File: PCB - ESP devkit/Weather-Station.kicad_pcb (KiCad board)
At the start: 2 copper layers, 61.5 x 50.5 mm, 28 parts, among them J1 Biruta, J10 Conn_01x19, J11 Conn_01x19, J2 Power, J3 BH1750-FVI, J4 BME280, J5 Pluviometro, J6 Anemometro, J8 Conn_01x02, J9 Conn_01x02, U1 AP1117-33

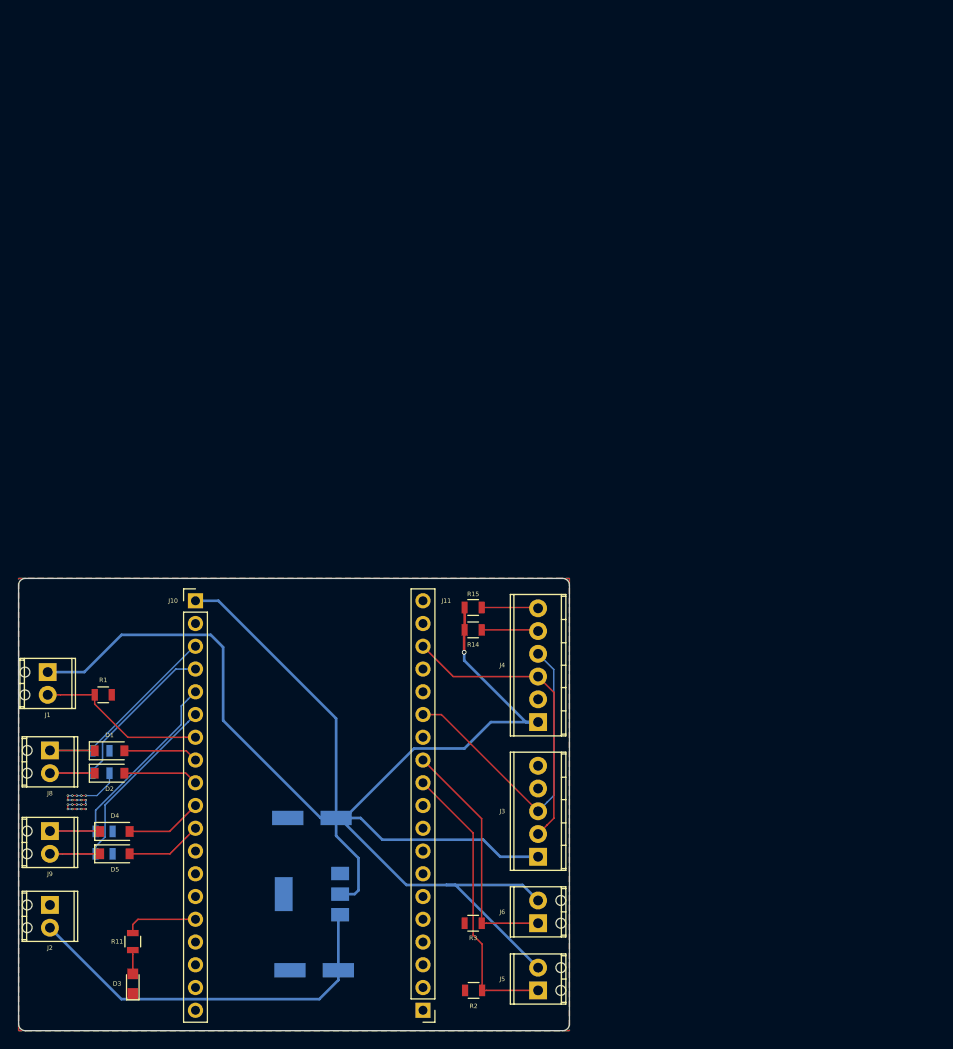
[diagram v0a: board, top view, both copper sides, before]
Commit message: Ajustando PCBs
Signed-off-by: Gustavo Costa <gustavocosta@ic.ufal.br>
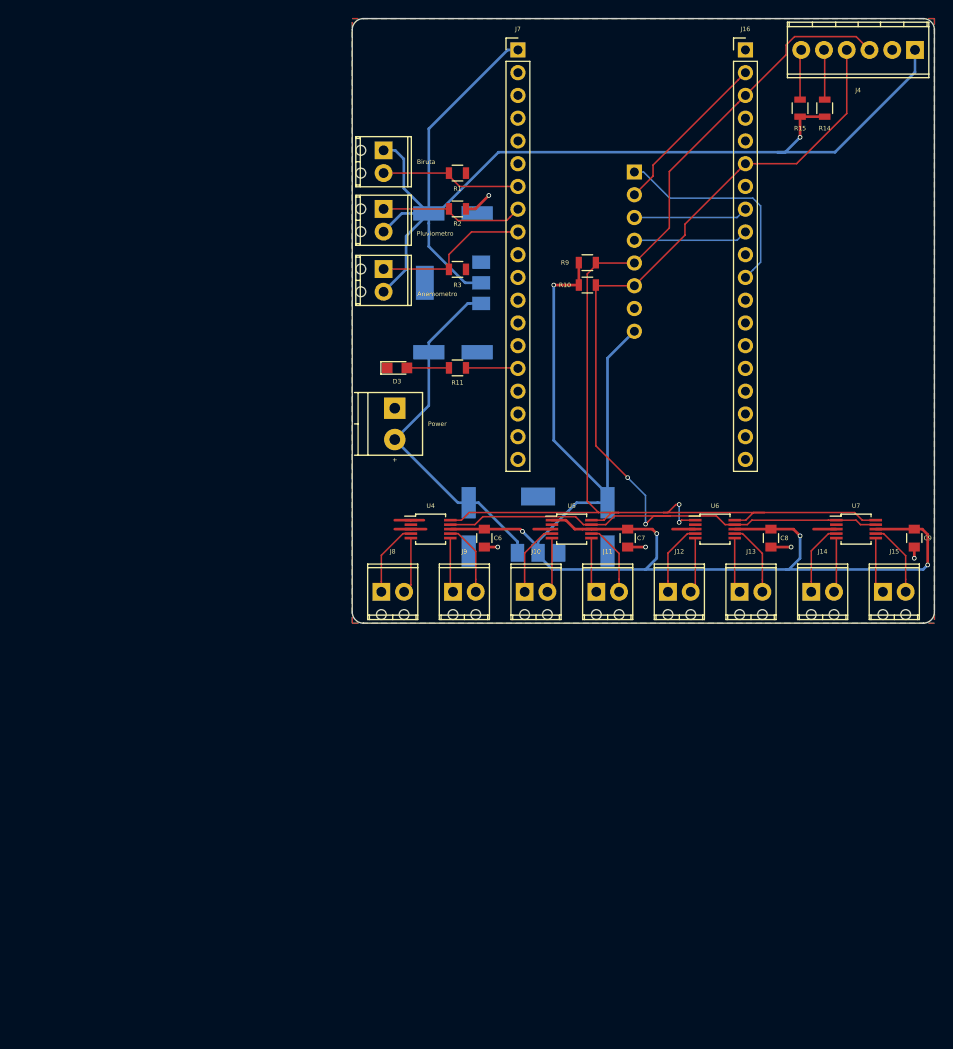
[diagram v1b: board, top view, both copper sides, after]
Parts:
- removed D1, D2, D4, D5: D, Diodes_SMD:D_SOD-123
- removed J1: Biruta, TerminalBlock_Phoenix:TerminalBlock_Phoenix_MPT-2.54mm_2pol
- removed J2: Power, TerminalBlock_Phoenix:TerminalBlock_Phoenix_MPT-2.54mm_2pol
- removed J5: Pluviometro, TerminalBlock_Phoenix:TerminalBlock_Phoenix_MPT-2.54mm_2pol
- removed J6: Anemometro, TerminalBlock_Phoenix:TerminalBlock_Phoenix_MPT-2.54mm_2pol
- removed R12, R13: 1.5K, Resistors_SMD:R_0805
- added Anemometro: Anemometro, TerminalBlock_Phoenix:TerminalBlock_Phoenix_MPT-2.54mm_2pol, F.Cu at (106.0, 55.5)
- added Biruta: Biruta, TerminalBlock_Phoenix:TerminalBlock_Phoenix_MPT-2.54mm_2pol, F.Cu at (106.0, 42.2)
- added C4: 22μF, Capacitors_SMD:CP_Elec_6.3x7.7, B.Cu at (115.5, 84.2)
- added C5: 22μF, Capacitors_SMD:CP_Elec_6.3x7.7, B.Cu at (131.0, 84.2)
- added C6: 0.1uF, Capacitors_SMD:C_0805, F.Cu at (117.2, 85.5)
- added C7: 0.1uF, Capacitors_SMD:C_0805, F.Cu at (133.2, 85.5)
- added C8: 0.1uF, Capacitors_SMD:C_0805, F.Cu at (149.2, 85.5)
- added C9: 0.1uF, Capacitors_SMD:C_0805, F.Cu at (165.2, 85.5)
- added J12: Conn_01x02, TerminalBlock_Phoenix:TerminalBlock_Phoenix_MPT-2.54mm_2pol, F.Cu at (137.8, 91.5)
- added J13: Conn_01x02, TerminalBlock_Phoenix:TerminalBlock_Phoenix_MPT-2.54mm_2pol, F.Cu at (145.8, 91.5)
- added J14: Conn_01x02, TerminalBlock_Phoenix:TerminalBlock_Phoenix_MPT-2.54mm_2pol, F.Cu at (153.8, 91.5)
- added J15: Conn_01x02, TerminalBlock_Phoenix:TerminalBlock_Phoenix_MPT-2.54mm_2pol, F.Cu at (161.8, 91.5)
- added J16: Conn_01x19, Pin_Headers:Pin_Header_Straight_1x19_Pitch2.54mm, F.Cu at (146.4, 31.0)
- added J7: Conn_01x19, Pin_Headers:Pin_Header_Straight_1x19_Pitch2.54mm, F.Cu at (121.0, 31.0)
- added Pluviometro: Pluviometro, TerminalBlock_Phoenix:TerminalBlock_Phoenix_MPT-2.54mm_2pol, F.Cu at (106.0, 48.8)
- added Power: Power, TerminalBlock_Phoenix:TerminalBlock_Phoenix_PT-3.5mm_2pol, F.Cu at (107.2, 71.0)
- added U3: AP1117-33, TO_SOT_Packages_SMD:SOT-223, B.Cu at (123.2, 84.0)
- added U4: ADS1115, Housings_SSOP:MSOP-10_3x3mm_Pitch0.5mm, F.Cu at (111.2, 84.5)
- added U5: ADS1115, Housings_SSOP:MSOP-10_3x3mm_Pitch0.5mm, F.Cu at (127.0, 84.5)
- added U6: ADS1115, Housings_SSOP:MSOP-10_3x3mm_Pitch0.5mm, F.Cu at (143.0, 84.5)
- added U7: ADS1115, Housings_SSOP:MSOP-10_3x3mm_Pitch0.5mm, F.Cu at (158.8, 84.5)
- J10, J11: value Conn_01x19 -> Conn_01x02; footprint Pin_Headers:Pin_Header_Straight_1x19_Pitch2.54mm -> TerminalBlock_Phoenix:TerminalBlock_Phoenix_MPT-2.54mm_2pol
- J3: value BH1750-FVI -> DataLogger; footprint TerminalBlock_Phoenix:TerminalBlock_Phoenix_MPT-2.54mm_5pol -> Pin_Headers:Pin_Header_Straight_1x08_Pitch2.54mm; moved to B.Cu
- R10, R9: value 1.5K -> 10k; moved to F.Cu
- moved R2 87.3 mm to (114.2, 48.8), turned to 180 degrees
- moved J4 86.0 mm to (165.3, 31.0), turned to 180 degrees
- moved J3 77.2 mm to (134.0, 44.6), turned to 180 degrees
- moved R10 76.9 mm to (128.8, 57.2)
- moved R9 76.9 mm to (128.8, 54.8)
- moved D3 74.8 mm to (107.5, 66.5), turned to 0 degrees
- moved R11 73.6 mm to (114.2, 66.5), turned to 180 degrees
- moved R3 73.0 mm to (114.2, 55.5), turned to 0 degrees
- moved C2 70.7 mm to (113.8, 64.8), turned to 0 degrees
- moved R1 70.4 mm to (114.2, 44.8)
- moved R14 70.2 mm to (155.2, 37.5), turned to 270 degrees
- moved U1 70.0 mm to (113.8, 57.0)
- moved C3 69.3 mm to (113.8, 49.2), turned to 0 degrees
- moved R15 66.6 mm to (152.5, 37.5), turned to 270 degrees
- moved J9 52.3 mm to (113.8, 91.5), turned to 0 degrees
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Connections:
- J10 pad 1: +3V3 -> Net-(J10-Pad1)
- J10 pad 2: (no net) -> Net-(J10-Pad2)
- J11 pad 1: (no net) -> Net-(J11-Pad1)
- J11 pad 2: (no net) -> Net-(J11-Pad2)
- J3 pad 1: +3V3 -> CS
- J3 pad 2: Net-(J11-Pad17) -> MOSI
- J3 pad 3: Net-(J11-Pad14) -> MISO
- J3 pad 4: (no net) -> SCK
- J3 pad 5: GND -> SCL
- J4 pad 3: Net-(J11-Pad17) -> SCL
- J4 pad 4: Net-(J11-Pad14) -> SDA
- J8 pad 1: ADC1_CH0 -> Net-(J8-Pad1)
- J8 pad 2: ADC1_CH3 -> Net-(J8-Pad2)
- J9 pad 1: ADC1_CH6 -> Net-(J9-Pad1)
- J9 pad 2: ADC1_CH7 -> Net-(J9-Pad2)
- R1 pad 1: ADC1_CH4 -> Net-(J1-Pad2)
- R10 pad 1: ADC1_CH3 -> +5V
- R10 pad 2: GND -> SDA
- R11 pad 1: Net-(J10-Pad15) -> Net-(J7-Pad15)
- R2 pad 2: Net-(J11-Pad11) -> Net-(J5-Pad1)
- R3 pad 1: Net-(J11-Pad12) -> Net-(J6-Pad1)
- R9 pad 1: ADC1_CH0 -> +5V
- R9 pad 2: GND -> SCL
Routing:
- net +5V: track 0.00 -> 157.6 mm, vias 0 -> 5
- net SCL: track 0.00 -> 136.1 mm, vias 0 -> 2
- net SDA: track 0.00 -> 125.4 mm, vias 0 -> 2
- net +3V3: track 200.5 -> 132.4 mm
- net Net-(J11-Pad14): track 36.4 -> 0.00 mm
- net Net-(J11-Pad17): track 33.3 -> 0.00 mm
- net Net-(J11-Pad11): track 32.2 -> 0.00 mm
- net ADC1_CH6: track 30.9 -> 0.00 mm
- net ADC1_CH7: track 30.9 -> 0.00 mm
- net Net-(J11-Pad12): track 27.2 -> 0.00 mm
- net ADC1_CH3: track 26.9 -> 0.00 mm
- net ADC1_CH0: track 25.8 -> 0.00 mm
- net CS: track 0.00 -> 24.4 mm
- net ADC1_CH4: track 19.1 -> 0.00 mm
- net MOSI: track 0.00 -> 18.8 mm
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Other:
- board size 61.5 x 50.5 mm -> 65 x 67.5 mm
- board text added: "+"
